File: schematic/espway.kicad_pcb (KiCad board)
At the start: 2 copper layers, 44.5 x 37 mm, 36 parts, among them J1 CONN_01X02, J2 CONN_01X02, J3 CONN_01X04_MALE, SW1 SW_Push, U1 LM1117-3.3, U2 ESP-12E, U3 DRV8835, U4 LSM6DS3

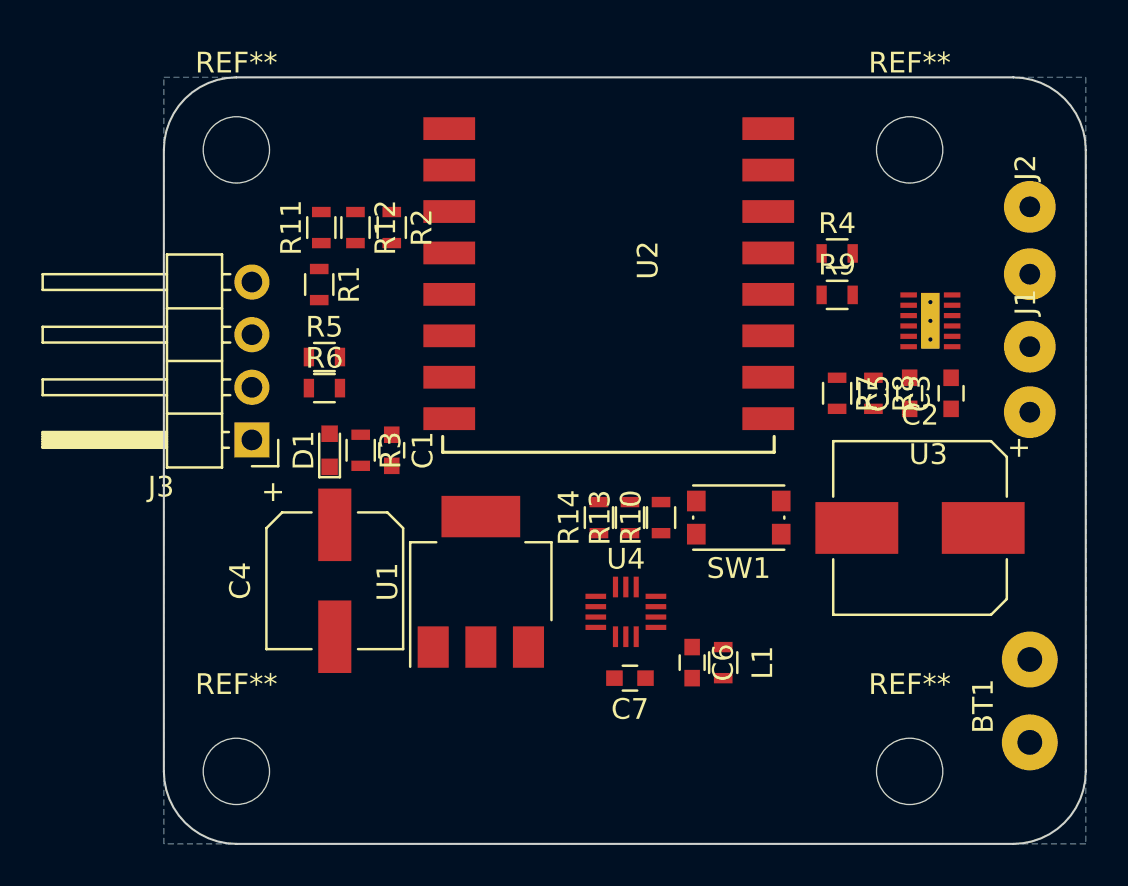
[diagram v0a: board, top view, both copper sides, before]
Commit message: PCB: stable checkpoint
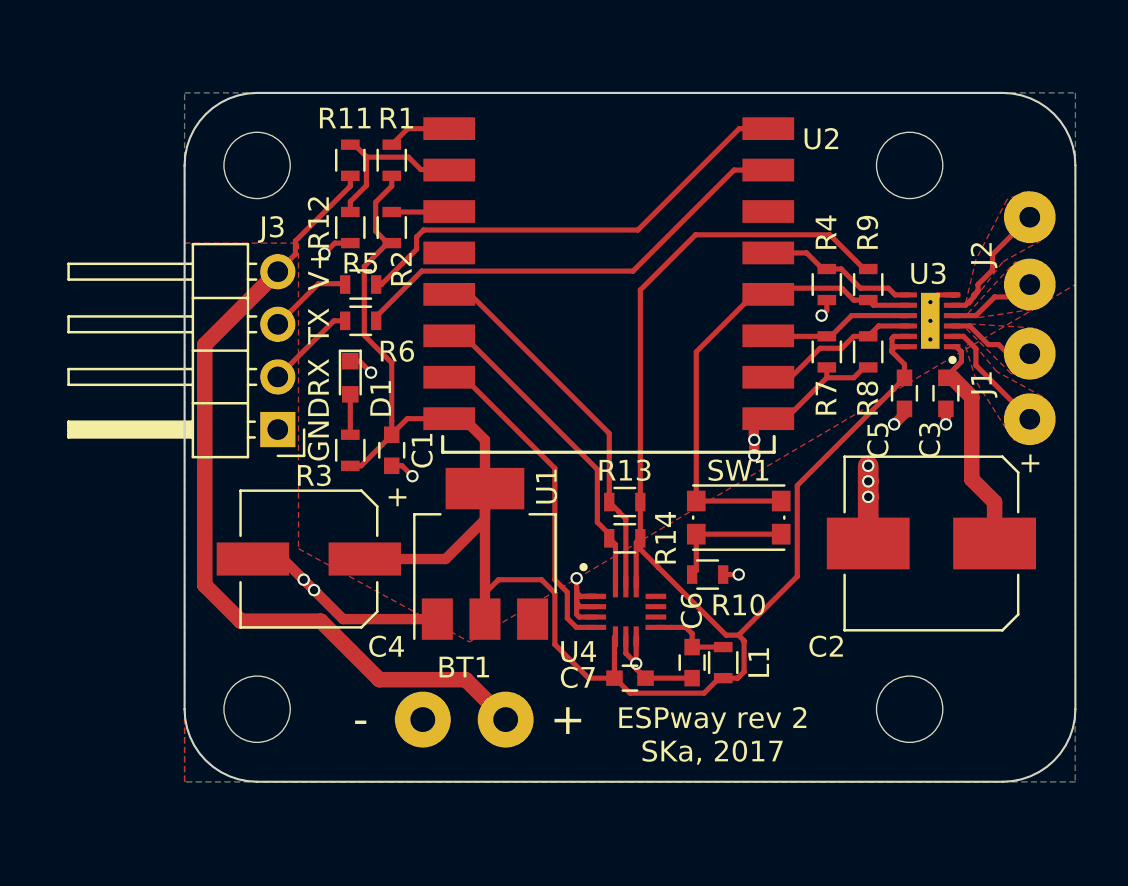
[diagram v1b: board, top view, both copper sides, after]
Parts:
- moved BT1 25.5 mm to (142.5, 151.5), turned to 180 degrees
- moved R1 6.95 mm to (137.0, 124.5)
- moved R5 3.91 mm to (135.5, 130.5)
- moved R6 3.69 mm to (135.5, 132.2)
- moved D1 3.64 mm to (135.0, 135.0), turned to 270 degrees
- moved R10 3.55 mm to (152.2, 144.5), turned to 0 degrees
- moved R11 3.54 mm to (135.0, 124.5)
- moved REF** 3.16 mm to (130.5, 151.0)
- moved REF** 3.00 mm to (162.0, 151.0)
- moved R7 2.06 mm to (158.0, 133.8)
- moved R8 2.02 mm to (160.0, 133.8)
- moved C4 1.63 mm to (133.0, 143.8), turned to 180 degrees
- moved R14 1.60 mm to (148.2, 142.8), turned to 180 degrees
- moved R4 1.58 mm to (158.0, 130.5), turned to 270 degrees
- moved R9 1.58 mm to (160.0, 130.5), turned to 270 degrees
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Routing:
- net +3V3: track 0.00 -> 115.1 mm
- net +BATT: track 0.00 -> 51.7 mm
- net GND: track 0.00 -> 45.2 mm, vias 0 -> 16
- net BPHASE: track 0.00 -> 23.2 mm
- net Net-(R5-Pad2): track 0.00 -> 21.8 mm
- net Net-(R6-Pad2): track 0.00 -> 21.7 mm
- net SCL: track 0.00 -> 17.6 mm
- net INT: track 0.00 -> 15.3 mm
- net SDA: track 0.00 -> 15.2 mm
- net ADC: track 0.00 -> 8.98 mm
- net APHASE: track 0.00 -> 8.50 mm
- net BENBL: track 0.00 -> 8.31 mm
- net AENBL: track 0.00 -> 7.90 mm
- net Net-(J2-Pad1): track 0.00 -> 6.18 mm
- net Net-(R10-Pad1): track 0.00 -> 6.13 mm
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- added copper zone on F.Cu, net +BATT
- added copper zone on F.Cu, net Net-(J1-Pad1)
- added copper zone on F.Cu, net Net-(J1-Pad2)
- added copper zone on F.Cu, net Net-(J2-Pad1)
- added copper zone on F.Cu, net Net-(J2-Pad2)
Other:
- board size 44.5 x 37 mm -> 43 x 33.2 mm
- board text added: "+"
- board text added: "-"
- board text added: "ESPway rev 2 SKa, 2017"
- board text added: "GND"
- board text added: "RX"
- board text added: "TX"
- board text added: "V+"
